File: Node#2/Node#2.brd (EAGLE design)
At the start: 60.5 x 120 mm, 135 parts, among them IC1 TSL25911FN, J1 68712414522, Q1 BC847ALT1SMD, Q2 SI1308EDL-T1-GE3, U2 RV8564C3, U3 BLUENRG-232, U4 TPS63001DRCT, Y3 ECS-160-12-36-AGN-TR, Y4 NX2012SA-32.768K-STD-MUB-1

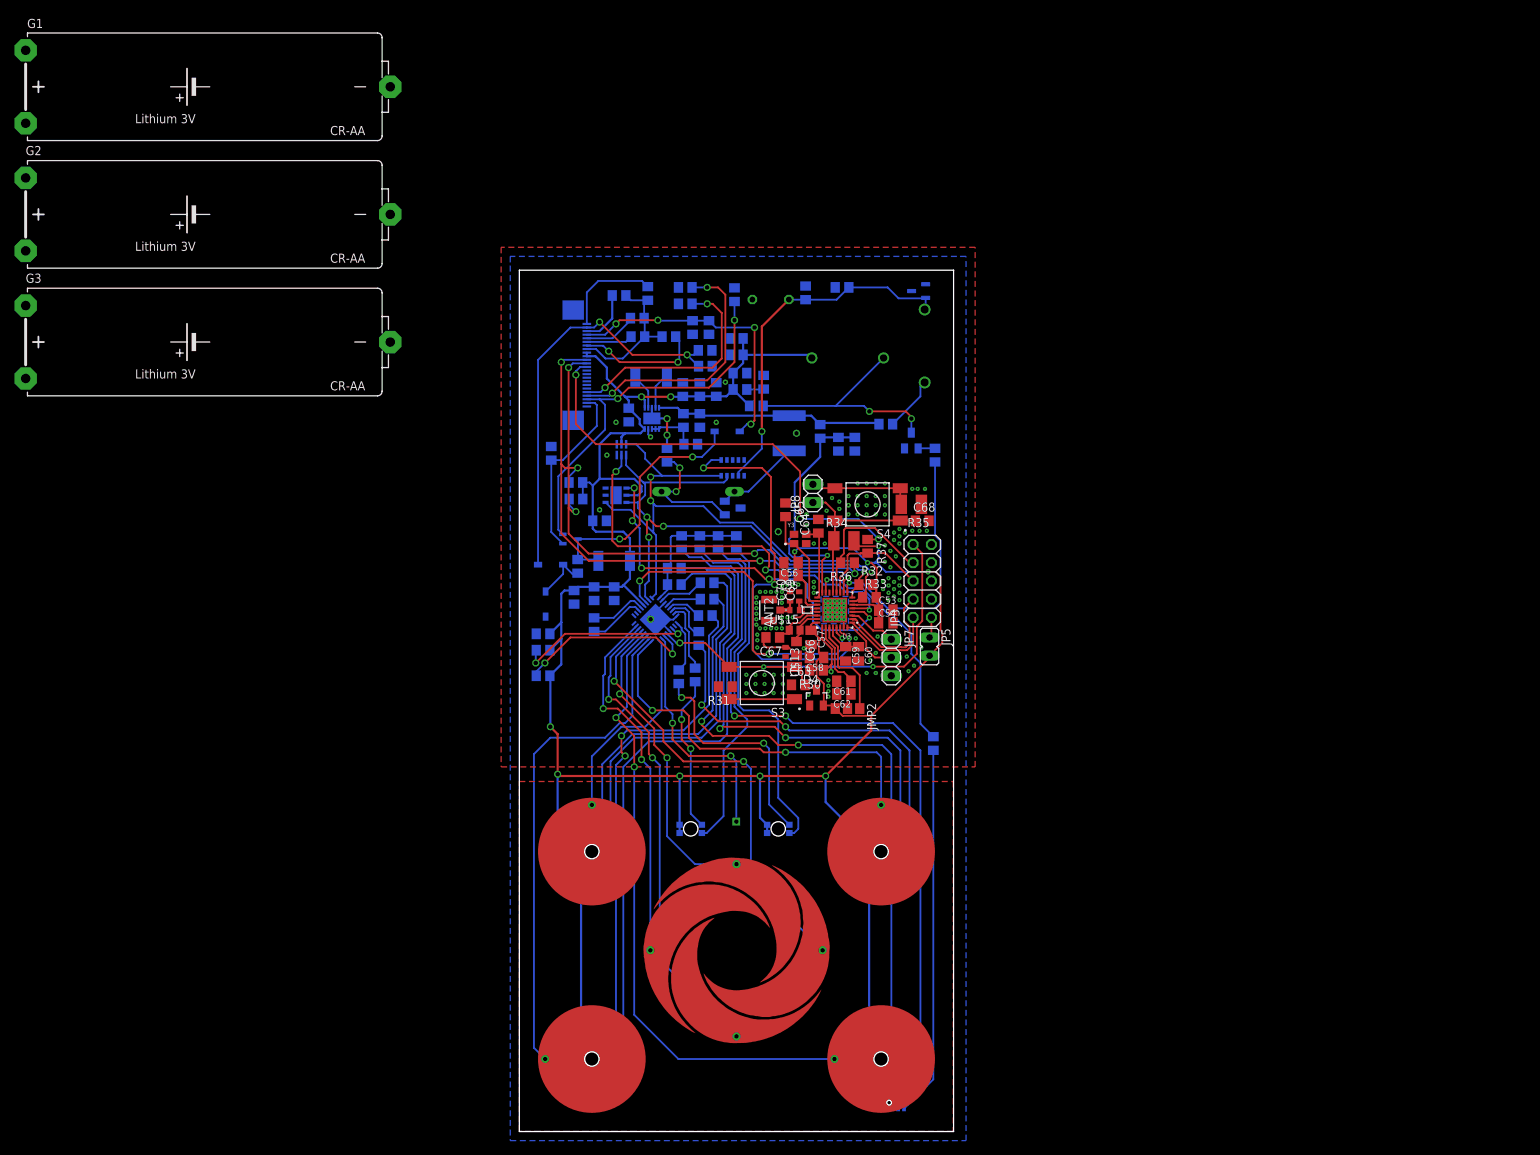
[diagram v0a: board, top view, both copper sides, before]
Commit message: Initial V2
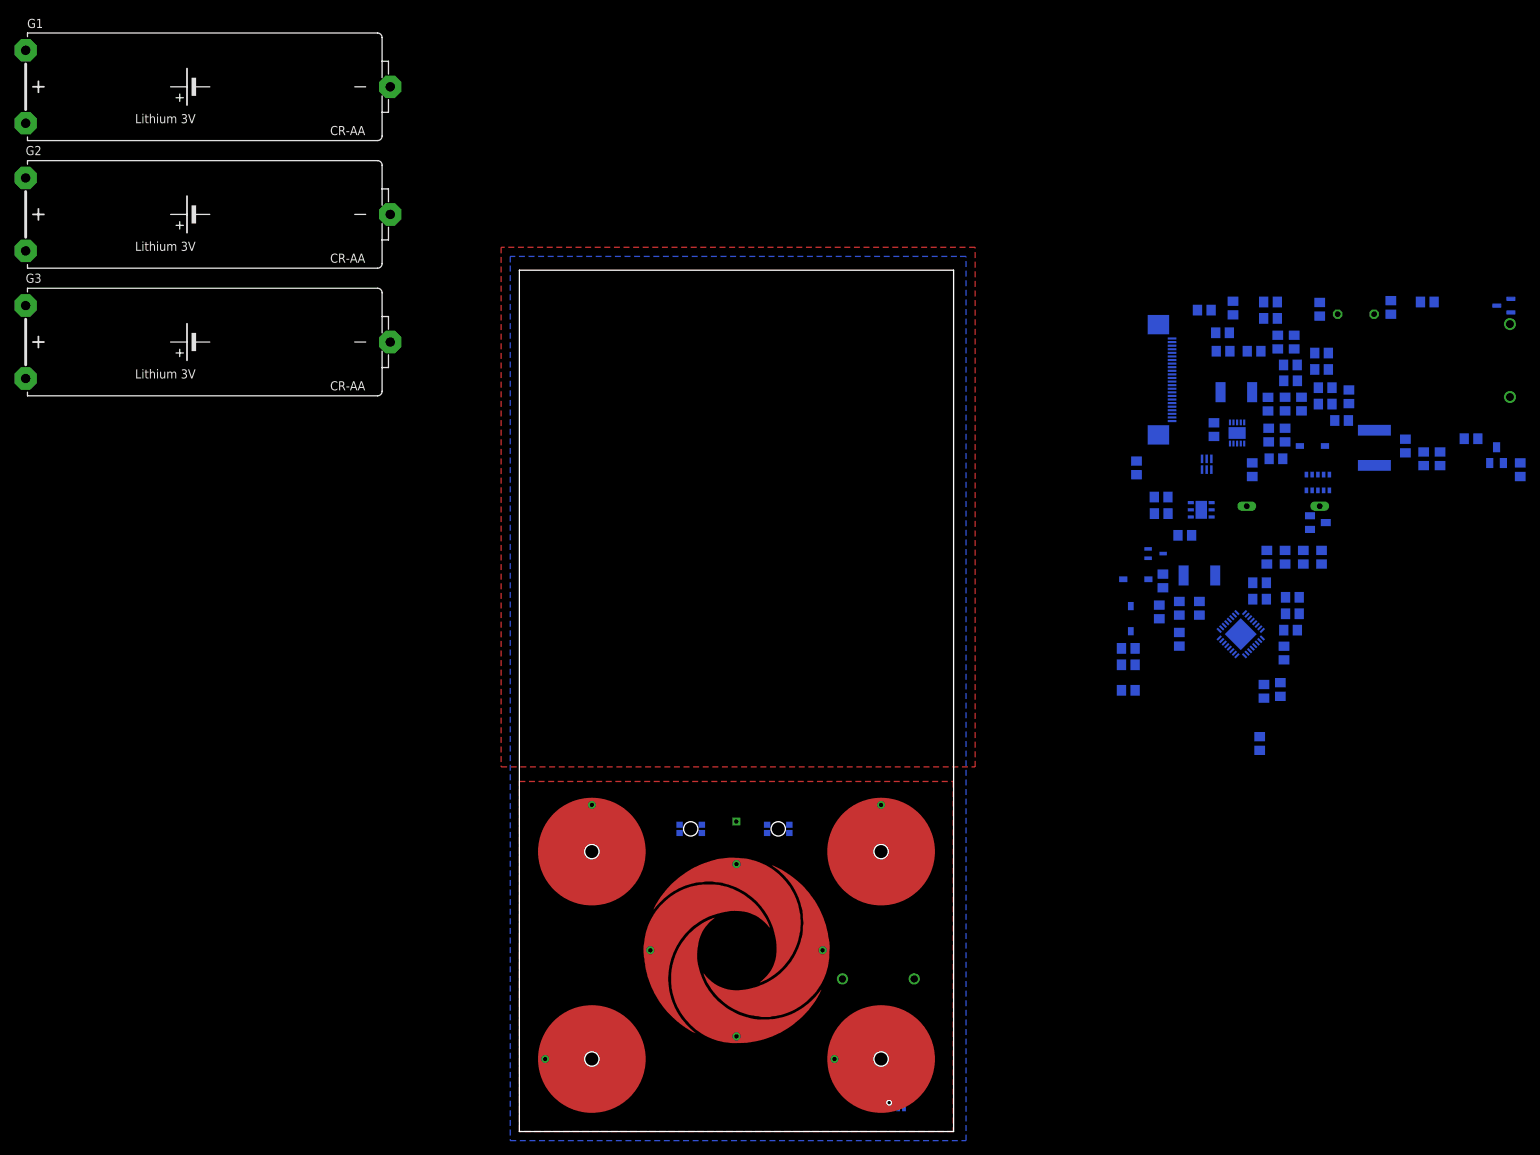
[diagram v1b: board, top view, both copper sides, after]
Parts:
- removed ANT2: CONUFL001-SMD, BlueHome:CONUFL001-SMD
- removed C53, C54, C55, C56, C57, C58, C59, C60, C61, C62: (no value), rcl:C0805K
- removed C63, C64, C65, C66, C67, C68: (no value), rcl:C0805
- removed C69, C70: (no value), rcl:C0402
- removed D4: BAS40-06, diode:SOT23
- removed JMP2: 0R-JUMPA, jump-0r-smd:A0R-JMP
- removed JP3: (no value), pinhead:2X05
- removed JP5: (no value), jumper:JP1
- removed JP7: (no value), pinhead:1X03
- removed JP8: (no value), pinhead:1X02
- removed R30, R31, R32, R33, R36, R37: (no value), rcl:R0805
- removed R34, R35: (no value), rcl:R1210
- removed S3, S4: FSM4JSMAATR, BlueHome:SW_FSM4JSMAATR
- removed U$13, U$15: L0402, BlueHome:R0402
- removed U$14: BALF-NRG-01D3, BlueHome:FLIPCHIP
- removed U3: BLUENRG-232, BlueHome:QFN50P500X500X100-33T345N
- removed Y3: ECS-160-12-36-AGN-TR, BlueHome:XTAL_ECS-160-12-36-AGN-TR
- removed Y4: NX2012SA-32.768K-STD-MUB-1, BlueHome:XTAL_NX2012SA-32.768K-STD-MUB-1
- R16: value 10k -> 0k
- moved LS1 86.6 mm to (50.0, 21.3), turned to 180 degrees
- moved C34 81.6 mm to (128.3, 93.7)
- moved C10 81.6 mm to (106.7, 97.0)
- moved C13 81.6 mm to (94.7, 72.9)
- moved C19 81.6 mm to (99.4, 114.7)
- moved C22 81.6 mm to (95.4, 114.4)
- moved C24 81.6 mm to (96.8, 97.8)
- moved C26 81.6 mm to (89.7, 76.7)
- moved C27 81.6 mm to (108.0, 110.0)
- moved C29 81.6 mm to (107.4, 106.8)
- moved C30 81.6 mm to (105.7, 110.0)
- moved C31 81.6 mm to (104.3, 101.3)
- moved C4 81.6 mm to (111.8, 108.5)
- moved C5 81.6 mm to (106.7, 101.3)
- moved C7 81.6 mm to (126.5, 115.6)
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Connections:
- removed net CS: R1.1, R18.2
- removed net DIO14: C68.1, JP8.1, R34.1, S4.1, S4.2, U3.13
- removed net JTCK: JP3.4, U3.2
- removed net JTMS: JP3.2, U3.1
- removed net N$48: C59.1, C60.1, U3.28
- removed net N$49: C61.1, C62.1, JMP2.2, U3.26
- removed net N$50: R31.1, S3.1, S3.2
- removed net N$51: C64.1, U3.17, Y3.3
- removed net N$52: C65.2, U3.18, Y3.1
- removed net N$53: C66.2, C67.2, U$13.1
- removed net N$54: C66.1, U3.23, Y4.2
- removed net N$55: C67.1, U3.22, Y4.1
- removed net N$56: C69.1, U$14.A1, U$15.1
- removed net N$57: ANT2.1, C70.1, U$15.2
- removed net N$58: JP3.1, JP5.1
- removed net N$59: JP8.2, R35.2, S4.3, S4.4
- removed net N$60: U$14.B1, U3.20
- removed net N$61: U$14.B2, U3.21
- removed net RXD: JP7.2, U3.32
- removed net SMPSFILT2: JMP2.1, U3.27
- removed net TDI: JP3.8, R36.2, U3.12
- removed net TDO: JP3.6, R37.2, U3.11
- removed net TXD: JP7.1, U3.3
- net +3V3: no longer C53.1, C54.1, C55.1, C56.1, C57.1, C58.1, D4.2, JMP2.3, JP5.2, R30.2, R32.2, R33.2, R34.2, U3.19, U3.24, U3.6
- net ADC1: no longer U3.15
- net ADC2: no longer U3.16
- net DIO0: no longer R36.1
- net DIO1: now also R1.1, R18.2; no longer R37.1
- net DIO12: no longer U3.30
- net DIO13: no longer U3.29
- net DIO2: no longer U3.10
- net DIO3: no longer U3.9
- net DIO6: no longer U3.5
- net DIO7: no longer U3.4
- net GND: no longer ANT2.2, ANT2.3, C53.2, C54.2, C55.2, C56.2, C57.2, C58.2, C59.2, C60.2, C61.2, C62.2, C63.1, C64.2, C65.1, C68.2, C69.2, C70.2, JP3.3, JP3.5, JP3.9, JP7.3, R31.2, R35.1, U$13.2, U$14.A2, U3.31, U3.33, Y3.2, Y3.4
- net RESETN: no longer C63.2, D4.3, JP3.10, R30.1, S3.3, S3.4, U3.25
- net SCL: no longer R32.1, U3.8
- net SDA: no longer R33.1, U3.7
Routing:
- net +3V3: track 400.9 -> 0.00 mm, vias 11 -> 0
- net N$27: track 102.5 -> 0.00 mm, vias 2 -> 0
- net N$7: track 91.6 -> 0.00 mm
- net N$32: track 86.0 -> 0.00 mm, vias 2 -> 0
- net N$30: track 84.0 -> 0.00 mm, vias 2 -> 0
- net SDA: track 83.0 -> 0.00 mm, vias 3 -> 0
- net DIO2: track 77.4 -> 0.00 mm, vias 4 -> 0
- net SCL: track 75.2 -> 0.00 mm, vias 4 -> 0
- net DIO0: track 73.4 -> 0.00 mm, vias 4 -> 0
- net N$13: track 73.3 -> 0.00 mm, vias 2 -> 0
- net RESETN: track 72.6 -> 0.00 mm, vias 4 -> 0
- net N$25: track 72.1 -> 0.00 mm, vias 2 -> 0
- net N$31: track 70.8 -> 0.00 mm
- net SEG3: track 66.6 -> 0.00 mm, vias 2 -> 0
- net DIO1: track 63.4 -> 0.00 mm, vias 3 -> 0
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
